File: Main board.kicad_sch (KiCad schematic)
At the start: 103 parts, among them CN1 PA001-6P, CN2 PA001-6P, J1 Conn_ARM_SWD_TagConnect_TC203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, J2 Conn_01x02_Pin, J3 Conn_01x02_Pin, J5 Connector, USB-TYPE-C-16P, J6 XT30UPB-F, J7 Conn_01x02_Pin, J8 Conn_01x04_Pin, Q1 SI7232DN-T1-GE3, Q2 SI7232DN-T1-GE3, SW1 SKRKAEE020, SW2 SKRKAEE020, SW3 SW_SPDT, SW4 SW_SPDT, U1 STM32U575VGTx, U10 TLV75733PDBV, U11 NRVB120VLSFT1G, U12 NRVB120VLSFT1G, U2 TPS62901RPJR, U7 SN74AHCT125DR, X1 1XXD32000MBA, Y1 ECS-327TXO-33-TR

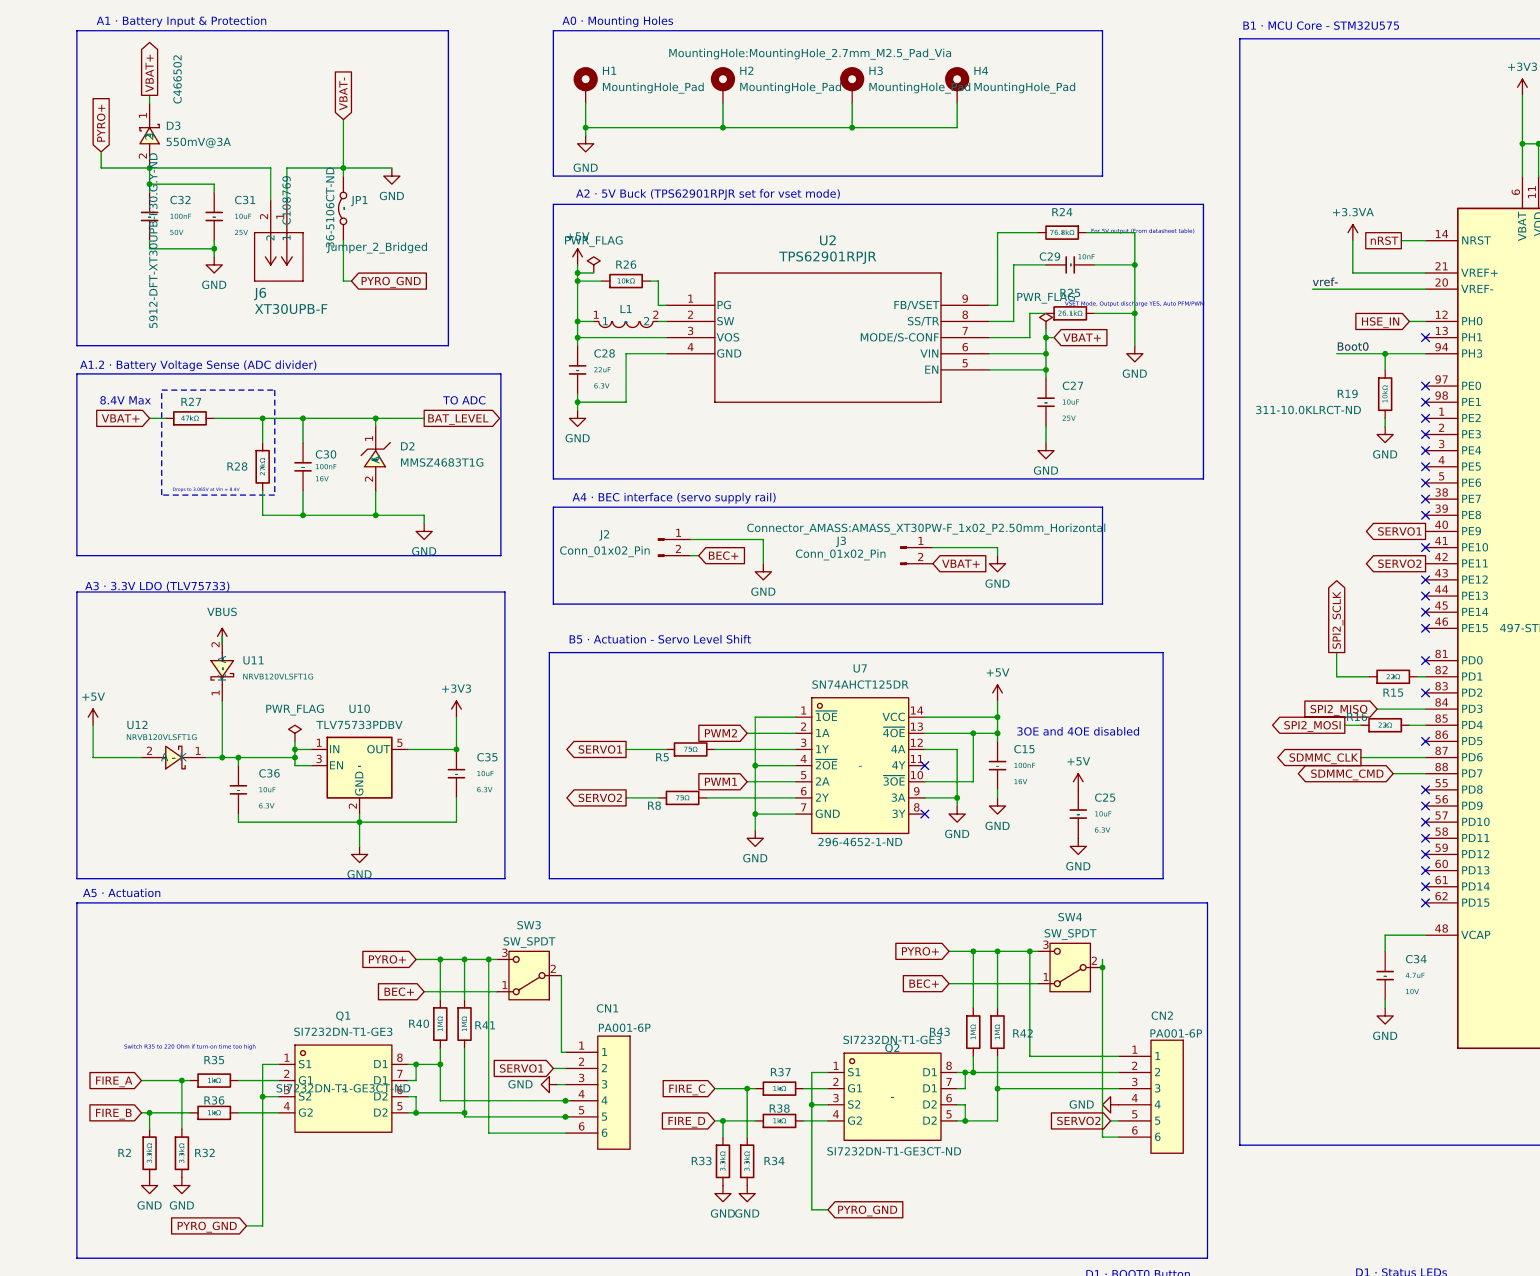
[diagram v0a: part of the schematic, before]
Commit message: New layout New.ioc
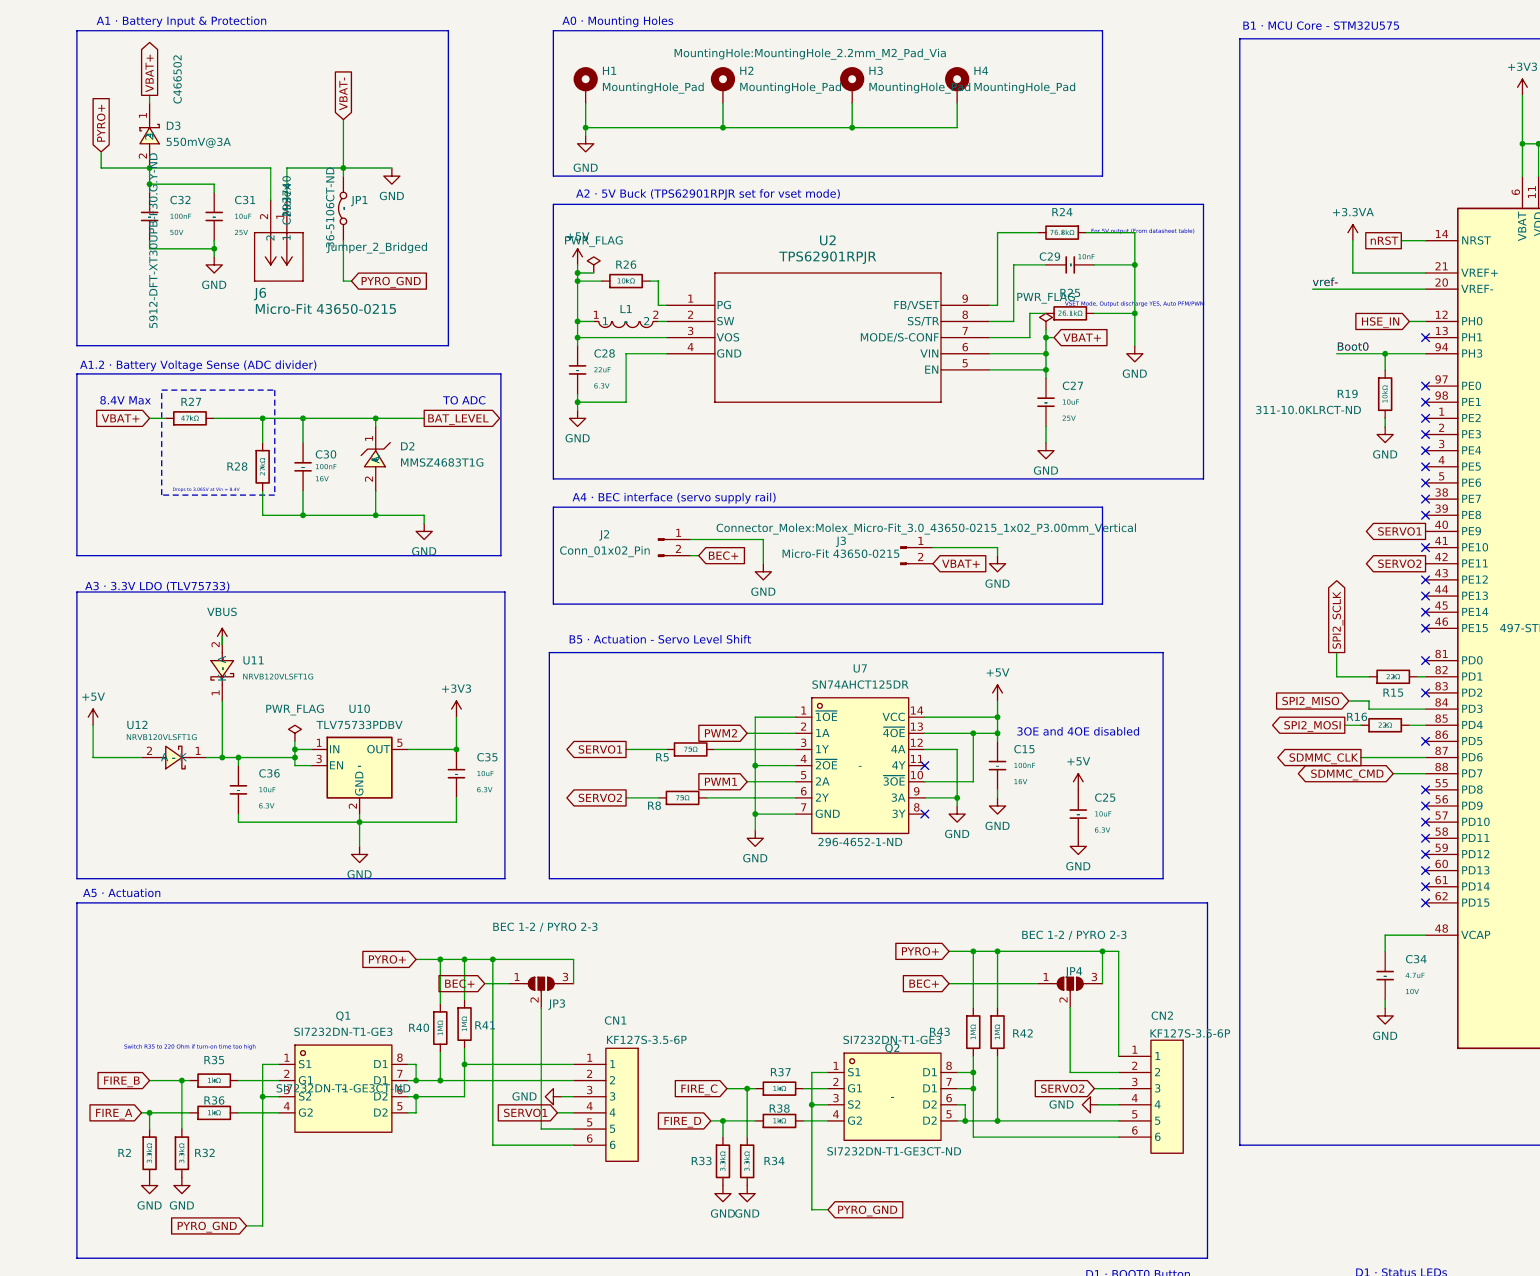
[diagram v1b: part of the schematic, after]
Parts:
- CN1, CN2: value PA001-6P -> KF127S-3.5-6P; footprint Mainboard_local:CONN-TH_6P-P5.00_PA001-6P -> TerminalBlock_Phoenix:TerminalBlock_Phoenix_PT-1,5-6-3.5-H_1x06_P3.50mm_Horizontal; LCSC Part C173288 -> C2974907; MPN PA001-6P -> KF127S-3.5-6P; Manufacturer 惠华 -> Cixi Kefa Elec
- H1, H2, H3, H4: footprint MountingHole:MountingHole_2.7mm_M2.5_Pad_Via -> MountingHole:MountingHole_2.2mm_M2_Pad_Via
- J3: value Conn_01x02_Pin -> Micro-Fit 43650-0215; footprint Connector_AMASS:AMASS_XT30PW-F_1x02_P2.50mm_Horizontal -> Connector_Molex:Molex_Micro-Fit_3.0_43650-0215_1x02_P3.00mm_Vertical; LCSC Part (none) -> C293740; MPN (none) -> 43650-0215
- J6: value XT30UPB-F -> Micro-Fit 43650-0215; footprint Connector_AMASS:AMASS_XT30UPB-F_1x02_P5.0mm_Vertical -> Connector_Molex:Molex_Micro-Fit_3.0_43650-0215_1x02_P3.00mm_Vertical; LCSC C108769 -> C293740; MANUFACTURER (none) -> Molex; MPN (none) -> 43650-0215
- JP3: renamed from SW3; value SW_SPDT -> BEC 1-2 / PYRO 2-3; footprint Mainboard_local:SW-TH_1101M2S3CQE2 -> Jumper:SolderJumper-3_P1.3mm_Open_Pad1.0x1.5mm_NumberLabels; symbol Switch:SW_SPDT -> Jumper:SolderJumper_3_Open; now left out of the parts list
- JP4: renamed from SW4; value SW_SPDT -> BEC 1-2 / PYRO 2-3; footprint Mainboard_local:SW-TH_1101M2S3CQE2 -> Jumper:SolderJumper-3_P1.3mm_Open_Pad1.0x1.5mm_NumberLabels; symbol Switch:SW_SPDT -> Jumper:SolderJumper_3_Open; now left out of the parts list
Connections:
- net FIRE_A: now also R2.1, R36.1; no longer R32.1, R35.1
- net FIRE_B: now also R32.1, R35.1; no longer R2.1, R36.1
- net SERVO1: now also CN1.4; no longer CN1.2
- net SERVO2: now also CN2.3; no longer CN2.5
- net at JP4.2 (C): now also CN2.2; no longer CN2.6
- net at JP3.2 (C): now also CN1.5; no longer CN1.1
- net at Q1.5 (D2), Q1.6 (D2), R41.2: now also CN1.1; no longer CN1.5
- net at Q1.7 (D1), Q1.8 (D1), R40.2: now also CN1.2; no longer CN1.4
- net at Q2.5 (D2), Q2.6 (D2), R42.2: now also CN2.5; no longer CN2.3
- net at Q2.7 (D1), Q2.8 (D1), R43.2: now also CN2.6; no longer CN2.2
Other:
- moved on the sheet: CN1, R40
